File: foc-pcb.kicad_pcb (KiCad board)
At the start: 4 copper layers, 32 x 32 mm, 88 parts, among them IC1 THVD2450VDRCR, Q1 CSD18540Q5B, Q2 CSD18540Q5B, Q7 CSD18540Q5B, Q8 CSD18540Q5B, U1 UCC272847, U10 TPS63070, U12 C2901617, U17 DF52-4S-0.8H(21), U18 DF52-4S-0.8H(21), U2 STM32G431CBT6, U3 INA241B4IDDFR, U5 RBB06DHHN, U6 SPX3819M5-L-5-0, U8 UCC272847, U9 INA241B4IDDFR

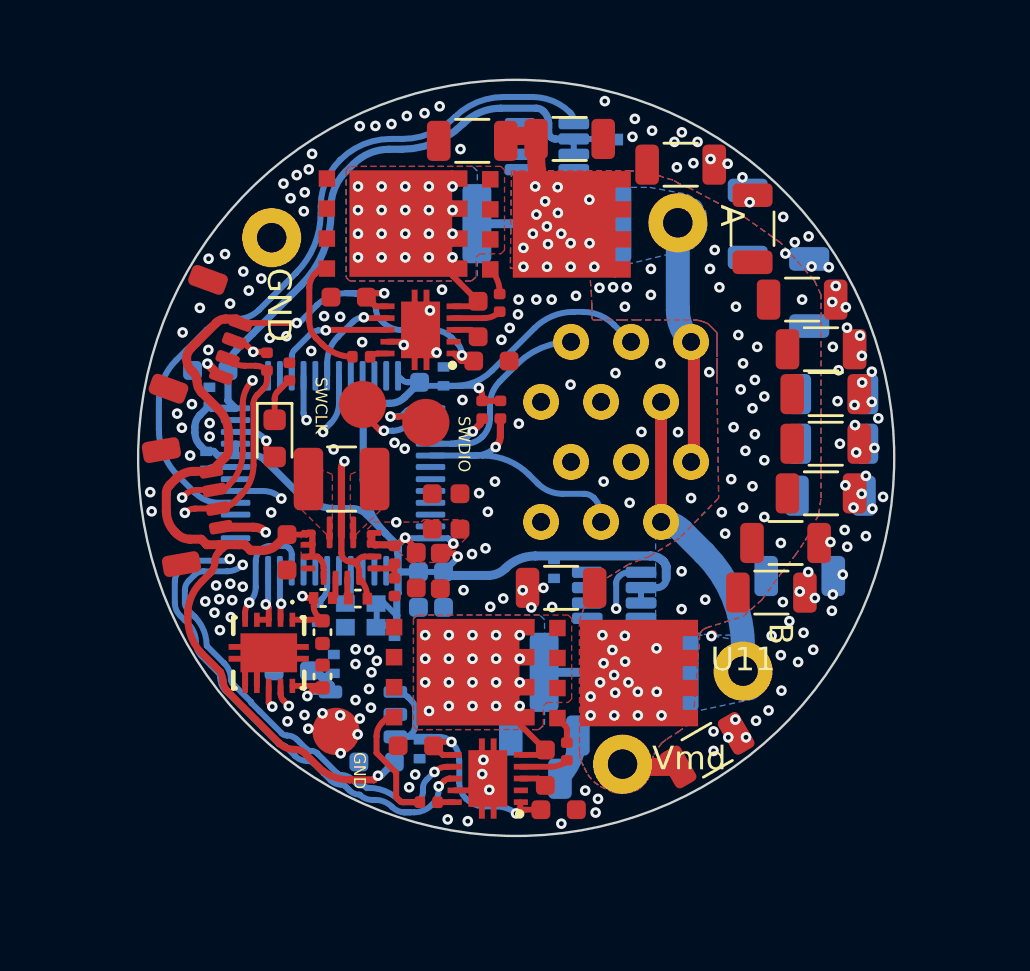
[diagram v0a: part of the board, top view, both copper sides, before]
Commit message: board clearance
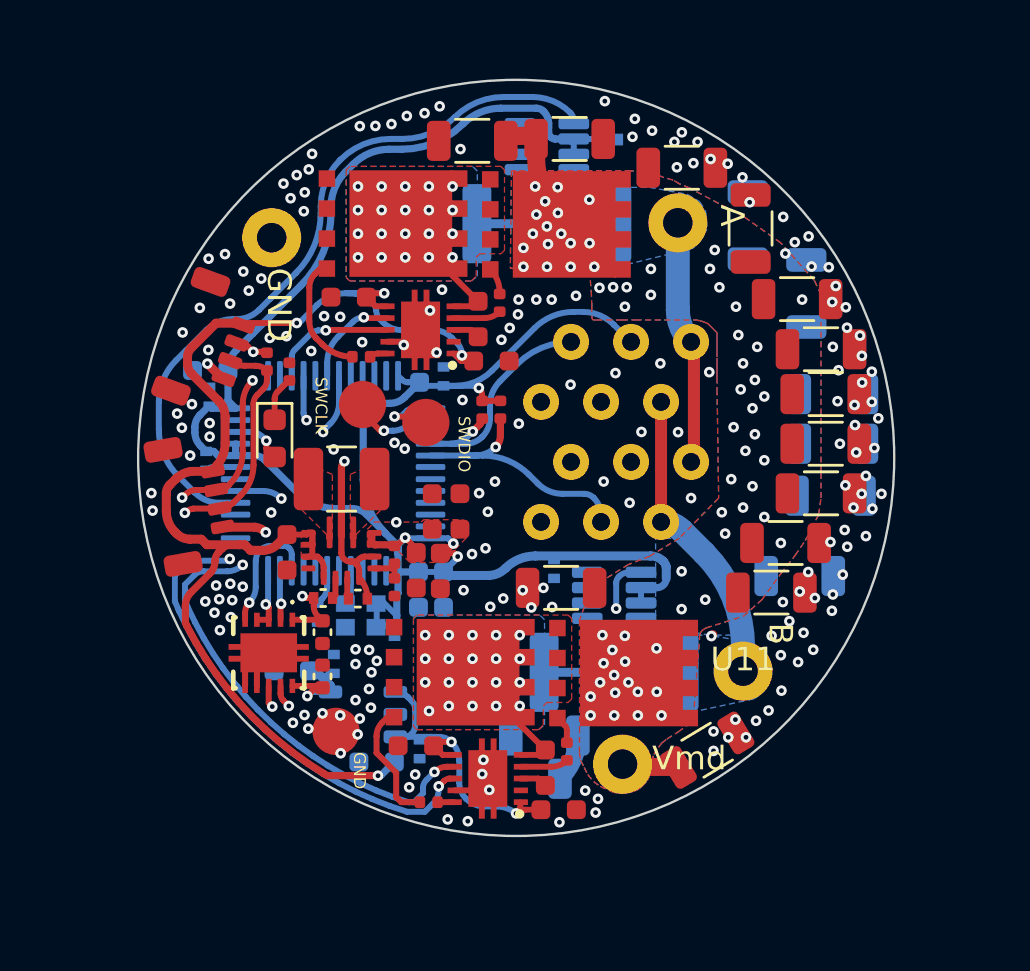
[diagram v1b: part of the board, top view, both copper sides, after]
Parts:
- moved C44 0.21 mm to (171.7, 127.3)
- moved C26 0.14 mm to (166.8, 121.7)
- moved U17 0.14 mm to (147.8, 129.5)
- moved C49 0.13 mm to (172.1, 127.0)
- moved C30 0.08 mm to (169.7, 124.3)
- moved U18 0.07 mm to (147.2, 135.7)
- moved C41 0.07 mm to (169.6, 124.2)
- turned C31 to 31 degrees
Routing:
- net /RS485/RS1_B: track 21.5 -> 22.1 mm
- net /STM32/TIM1_CH2N: track 29.8 -> 29.2 mm
